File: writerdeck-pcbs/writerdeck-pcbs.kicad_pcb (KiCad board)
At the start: 2 copper layers, 1 x 0.7 mm, 5 parts, among them J1 USB_C_Receptacle, J2 12401826E412A, U1 RP2040, U2 BQ25792RQMR

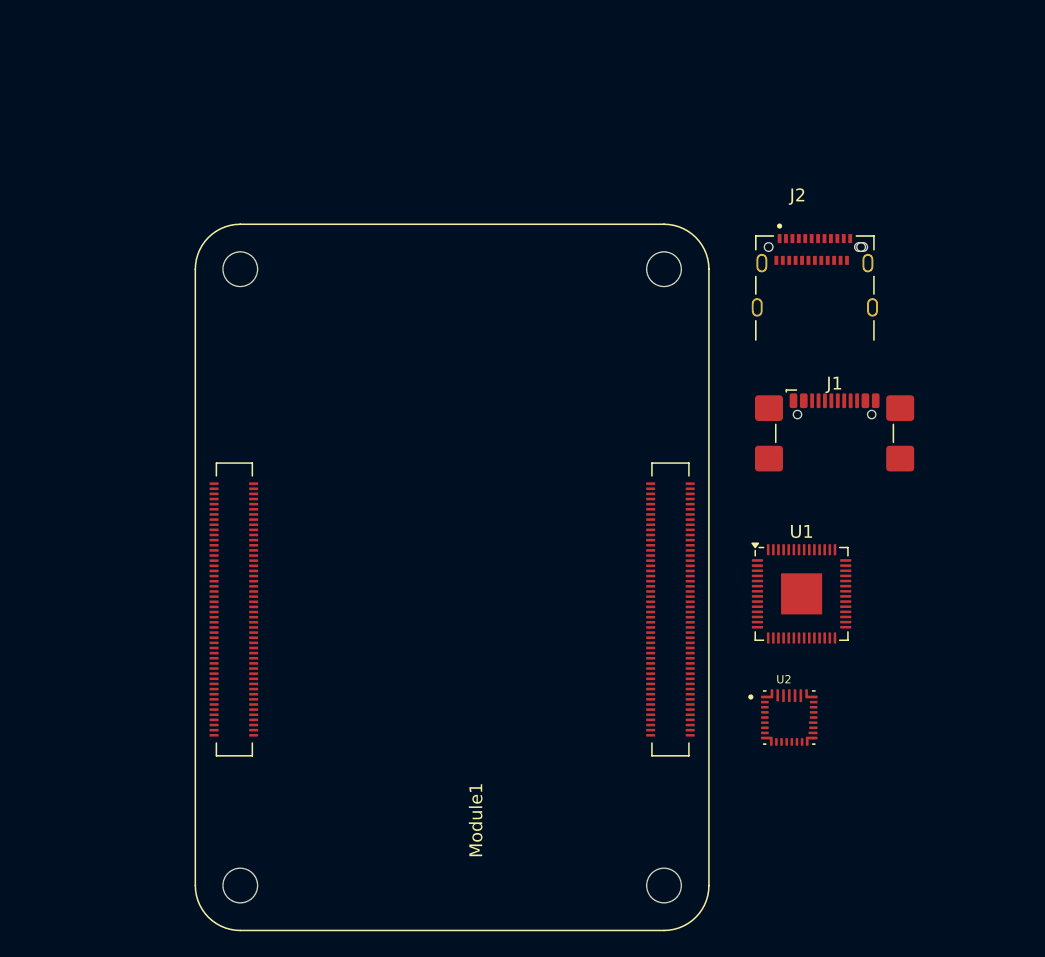
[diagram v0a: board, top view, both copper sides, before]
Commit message: power management done
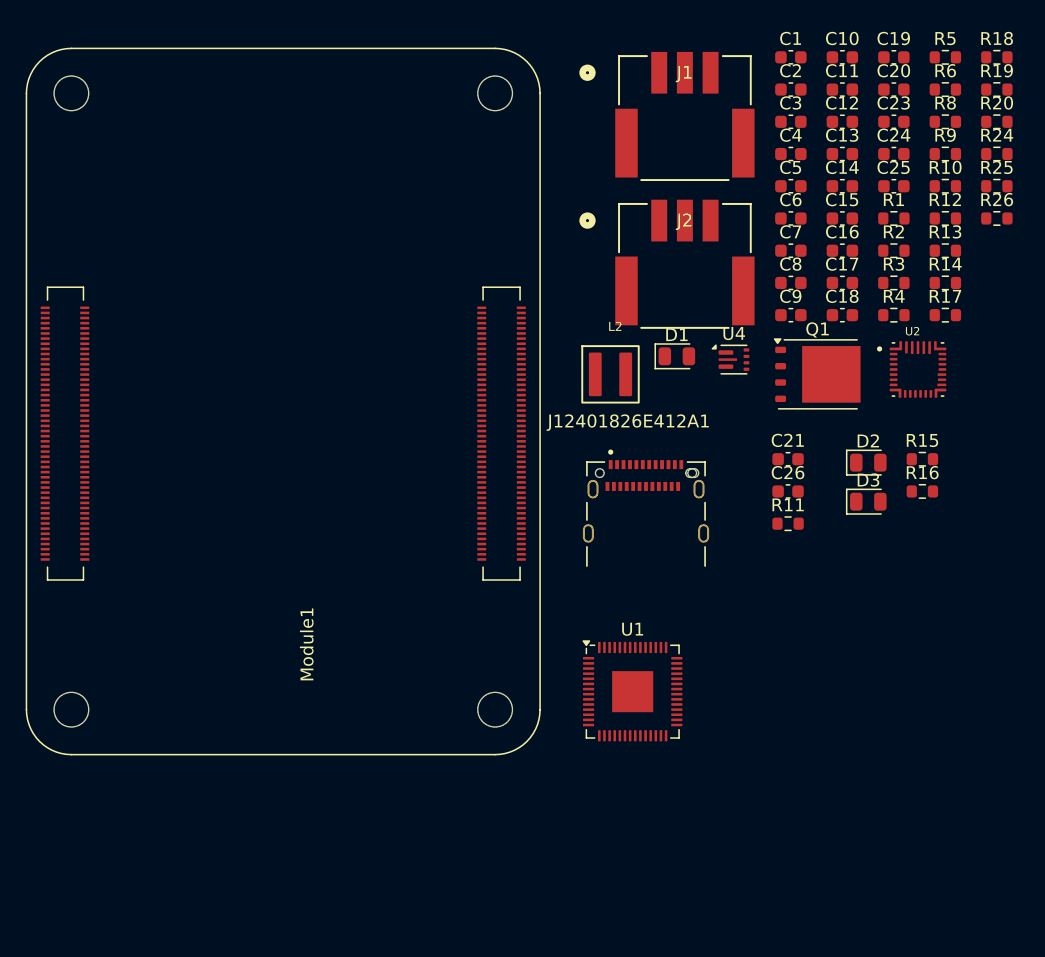
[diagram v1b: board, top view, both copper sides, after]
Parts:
- added C1: 10u, Capacitor_SMD:C_0603_1608Metric, F.Cu at (74.4, 17.5)
- added C10: 10u, Capacitor_SMD:C_0603_1608Metric, F.Cu at (78.4, 17.5)
- added C11: 10u, Capacitor_SMD:C_0603_1608Metric, F.Cu at (78.4, 20.0)
- added C12: 47n, Capacitor_SMD:C_0603_1608Metric, F.Cu at (78.4, 22.5)
- added C13: 47n, Capacitor_SMD:C_0603_1608Metric, F.Cu at (78.4, 25.0)
- added C14: 100n, Capacitor_SMD:C_0603_1608Metric, F.Cu at (78.4, 27.5)
- added C15: 10u, Capacitor_SMD:C_0603_1608Metric, F.Cu at (78.4, 30.1)
- added C16: 10u, Capacitor_SMD:C_0603_1608Metric, F.Cu at (78.4, 32.6)
- added C17: 10u, Capacitor_SMD:C_0603_1608Metric, F.Cu at (78.4, 35.1)
- added C18: 10u, Capacitor_SMD:C_0603_1608Metric, F.Cu at (78.4, 37.6)
- added C19: 10u, Capacitor_SMD:C_0603_1608Metric, F.Cu at (82.4, 17.5)
- added C2: 22u, Capacitor_SMD:C_0603_1608Metric, F.Cu at (74.4, 20.0)
- added C20: 10u, Capacitor_SMD:C_0603_1608Metric, F.Cu at (82.4, 20.0)
- added C21: 100n, Capacitor_SMD:C_0603_1608Metric, F.Cu at (74.2, 48.8)
- added C23: 10u, Capacitor_SMD:C_0603_1608Metric, F.Cu at (82.4, 22.5)
- added C24: 22u, Capacitor_SMD:C_0603_1608Metric, F.Cu at (82.4, 25.0)
- added C25: 22u, Capacitor_SMD:C_0603_1608Metric, F.Cu at (82.4, 27.5)
- added C26: 100n, Capacitor_SMD:C_0603_1608Metric, F.Cu at (74.2, 51.3)
- added C3: 4u7, Capacitor_SMD:C_0603_1608Metric, F.Cu at (74.4, 22.5)
- added C4: 100n, Capacitor_SMD:C_0603_1608Metric, F.Cu at (74.4, 25.0)
- added C5: 10u, Capacitor_SMD:C_0603_1608Metric, F.Cu at (74.4, 27.5)
- added C6: 10u, Capacitor_SMD:C_0603_1608Metric, F.Cu at (74.4, 30.1)
- added C7: 2u2, Capacitor_SMD:C_0603_1608Metric, F.Cu at (74.4, 32.6)
- added C8: 100n, Capacitor_SMD:C_0603_1608Metric, F.Cu at (74.4, 35.1)
- added C9: 10u, Capacitor_SMD:C_0603_1608Metric, F.Cu at (74.4, 37.6)
- added D1: Blue LED, LED_SMD:LED_0805_2012Metric, F.Cu at (65.5, 40.8)
- added D2: Red LED, LED_SMD:LED_0805_2012Metric, F.Cu at (80.4, 49.1)
- added D3: Green LED, LED_SMD:LED_0805_2012Metric, F.Cu at (80.4, 52.1)
- added J12401826E412A1: USB_C_Receptacle, ZF_common:12401826E412A, F.Cu at (63.1, 53.5)
- added L2: 1u, ZF_common:XFL4020-102MEC, F.Cu at (60.3, 42.2)
- added Q1: CSD17575Q3, Package_TO_SOT_SMD:TDSON-8-1, F.Cu at (76.5, 42.2)
- added R1: 2, Resistor_SMD:R_0603_1608Metric, F.Cu at (82.4, 30.1)
- added R10: 10k, Resistor_SMD:R_0603_1608Metric, F.Cu at (86.4, 27.5)
- added R11: 2k2, Resistor_SMD:R_0603_1608Metric, F.Cu at (74.2, 53.8)
- added R12: 100, Resistor_SMD:R_0603_1608Metric, F.Cu at (86.4, 30.1)
- added R13: 10k, Resistor_SMD:R_0603_1608Metric, F.Cu at (86.4, 32.6)
- added R14: 100k, Resistor_SMD:R_0603_1608Metric, F.Cu at (86.4, 35.1)
- added R15: 1k, Resistor_SMD:R_0603_1608Metric, F.Cu at (84.6, 48.8)
- added R16: 1k, Resistor_SMD:R_0603_1608Metric, F.Cu at (84.6, 51.3)
- added R17: 10k, Resistor_SMD:R_0603_1608Metric, F.Cu at (86.4, 37.6)
- added R18: 100k, Resistor_SMD:R_0603_1608Metric, F.Cu at (90.4, 17.5)
- added R19: 732k, Resistor_SMD:R_0603_1608Metric, F.Cu at (90.4, 20.0)
- added R2: 10k, Resistor_SMD:R_0603_1608Metric, F.Cu at (82.4, 32.6)
- added R20: 620, Resistor_SMD:R_0603_1608Metric, F.Cu at (90.4, 22.5)
- added R24: 15k, Resistor_SMD:R_0603_1608Metric, F.Cu at (90.4, 25.0)
- added R25: 100, Resistor_SMD:R_0603_1608Metric, F.Cu at (90.4, 27.5)
- added R26: 50, Resistor_SMD:R_0603_1608Metric, F.Cu at (90.4, 30.1)
- added R3: 3k, Resistor_SMD:R_0603_1608Metric, F.Cu at (82.4, 35.1)
- added R4: 10k, Resistor_SMD:R_0603_1608Metric, F.Cu at (82.4, 37.6)
- added R5: 300k, Resistor_SMD:R_0603_1608Metric, F.Cu at (86.4, 17.5)
- added R6: 2k2, Resistor_SMD:R_0603_1608Metric, F.Cu at (86.4, 20.0)
- added R8: 2k, Resistor_SMD:R_0603_1608Metric, F.Cu at (86.4, 22.5)
- added R9: 10k, Resistor_SMD:R_0603_1608Metric, F.Cu at (86.4, 25.0)
- added U4: TPS61022, Package_DFN_QFN:Texas_RWU0007A_VQFN-7_2x2mm_P0.5mm, F.Cu at (69.9, 41.0)
- J1: value USB_C_Receptacle -> 5023520300; footprint Connector_USB:USB_C_Receptacle_GCT_USB4110 -> ZF_common:5023520300
- J2: value 12401826E412A -> 5023520300; footprint ZF_common:12401826E412A -> ZF_common:5023520300
- moved U2 28.9 mm to (84.3, 41.8)
- moved J1 28.2 mm to (66.1, 22.2)
- moved Module1 19.0 mm to (18.3, 68.3)
- moved U1 15.2 mm to (62.1, 66.9)
- moved J2 10.3 mm to (66.1, 33.7)
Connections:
- Module1 pad 21: unconnected-(Module1A-LED_nACT-Pad21) -> /Base/CM5 GPIO/LED_nACT
- Module1 pad 92: unconnected-(Module1A-PWR_BUT-Pad92) -> PWR_BUT
- Module1 pad 95: unconnected-(Module1A-LED_nPWR-Pad95) -> /Base/CM5 GPIO/LED_nPWR
- U2 pad 1: unconnected-(U2-STAT-Pad1) -> /Base/Power Management/STAT
- U2 pad 10: unconnected-(U2-ACDRV2-Pad10) -> GND
- U2 pad 11: unconnected-(U2-ACDRV1-Pad11) -> GND
- U2 pad 12: unconnected-(U2-~{QON}-Pad12) -> PWR_BUT
- U2 pad 13: unconnected-(U2-~{CE}-Pad13) -> Net-(U2-~{CE})
- U2 pad 14: unconnected-(U2-SCL-Pad14) -> Net-(U2-SCL)
- U2 pad 15: unconnected-(U2-SDA-Pad15) -> Net-(U2-SDA)
- U2 pad 16: unconnected-(U2-TS-Pad16) -> /Base/Power Management/BATT_TEMP
- U2 pad 17: unconnected-(U2-ILIM_HIZ-Pad17) -> /Base/Power Management/ILIM_HIZ
- U2 pad 18: unconnected-(U2-BATP-Pad18) -> /Base/Power Management/BATP
- U2 pad 19: unconnected-(U2-BTST2-Pad19) -> /Base/Power Management/BTST2
- U2 pad 2: unconnected-(U2-VBUS-Pad2) -> VBUS
- U2 pad 20: unconnected-(U2-PROG-Pad20) -> Net-(U2-PROG)
- U2 pad 21: unconnected-(U2-~{INT}-Pad21) -> Net-(U2-~{INT})
- U2 pad 22: unconnected-(U2-BAT-Pad22) -> /Base/Power Management/BAT
- U2 pad 23: unconnected-(U2-BAT__1-Pad23) -> /Base/Power Management/BAT
- U2 pad 24: unconnected-(U2-SDRV-Pad24) -> /Base/Power Management/SDRV
- U2 pad 25: unconnected-(U2-SYS-Pad25) -> /Base/Power Management/VSYS
- U2 pad 26: unconnected-(U2-SW2-Pad26) -> /Base/Power Management/SW2
- U2 pad 27: unconnected-(U2-GND-Pad27) -> GND
- U2 pad 28: unconnected-(U2-SW1-Pad28) -> /Base/Power Management/SW1
- U2 pad 29: unconnected-(U2-PMID-Pad29) -> Net-(U2-PMID)
- U2 pad 3: unconnected-(U2-VBUS__1-Pad3) -> VBUS
- U2 pad 4: unconnected-(U2-BTST1-Pad4) -> /Base/Power Management/BTST1
- U2 pad 5: unconnected-(U2-REGN-Pad5) -> /Base/Power Management/REGN
- U2 pad 6: /Base/Power Management/USB2_P -> /Base/USB2_P
- U2 pad 7: /Base/Power Management/USB2_N -> /Base/USB2_N
- U2 pad 8: unconnected-(U2-VAC2-Pad8) -> VBUS
- U2 pad 9: unconnected-(U2-VAC1-Pad9) -> VBUS
